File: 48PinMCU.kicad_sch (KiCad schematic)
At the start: 34 parts, among them J5 SWD_Header, J6 SWD, SW1 Reset, SW2 SW_SPDT, U2 STM32G473CETx, Y1 Crystal

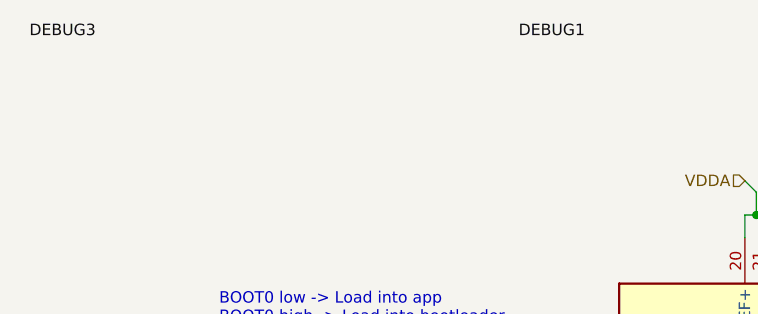
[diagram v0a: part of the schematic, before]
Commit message: layout placing
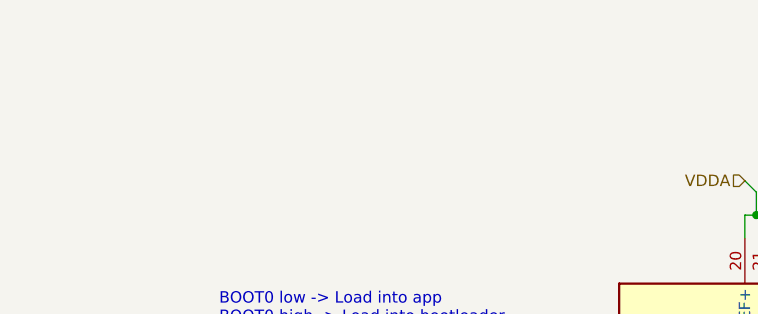
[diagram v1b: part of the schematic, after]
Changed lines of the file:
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@@
-		)
-	)
-	(label "DEBUG3"
-		(at 7.8802 2.0957 180)
-		(effects
-			(font
-				(size 1.27 1.27)
-			)
-			(justify right bottom)
 		)
 	)
@@
 		(effects
 			(font
-				(size 1.27 1.27)
-			)
-			(justify left bottom)
-		)
-	)
-	(label "DEBUG1"
-		(at 54.8702 2.0957 0)
-		(effects
-			(font

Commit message: not pretty
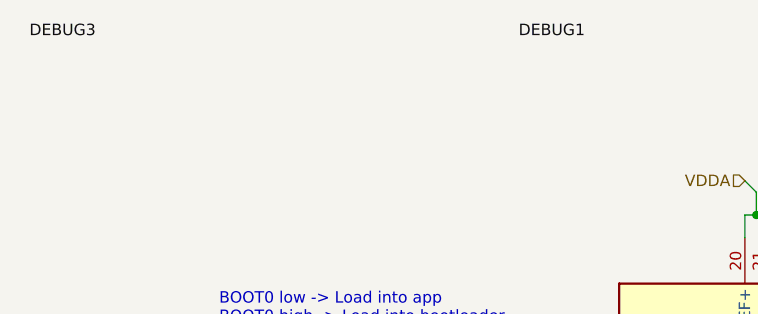
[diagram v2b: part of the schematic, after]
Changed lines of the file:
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@@
+		)
+	)
+	(label "DEBUG3"
+		(at 7.8802 2.0957 180)
+		(effects
+			(font
+				(size 1.27 1.27)
+			)
+			(justify right bottom)
 		)
 	)
@@
 		(effects
 			(font
+				(size 1.27 1.27)
+			)
+			(justify left bottom)
+		)
+	)
+	(label "DEBUG1"
+		(at 54.8702 2.0957 0)
+		(effects
+			(font
